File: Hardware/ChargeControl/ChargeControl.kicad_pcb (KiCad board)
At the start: 2 copper layers, 57 x 28 mm, 28 parts, among them J1 Conn_01x03, J2 Conn_01x04, J3 Conn_01x04, J4 Conn_01x08, Q1 Q-FET-N-SSM3K36MFV, U1 74LVC1G14, U2 MCP602

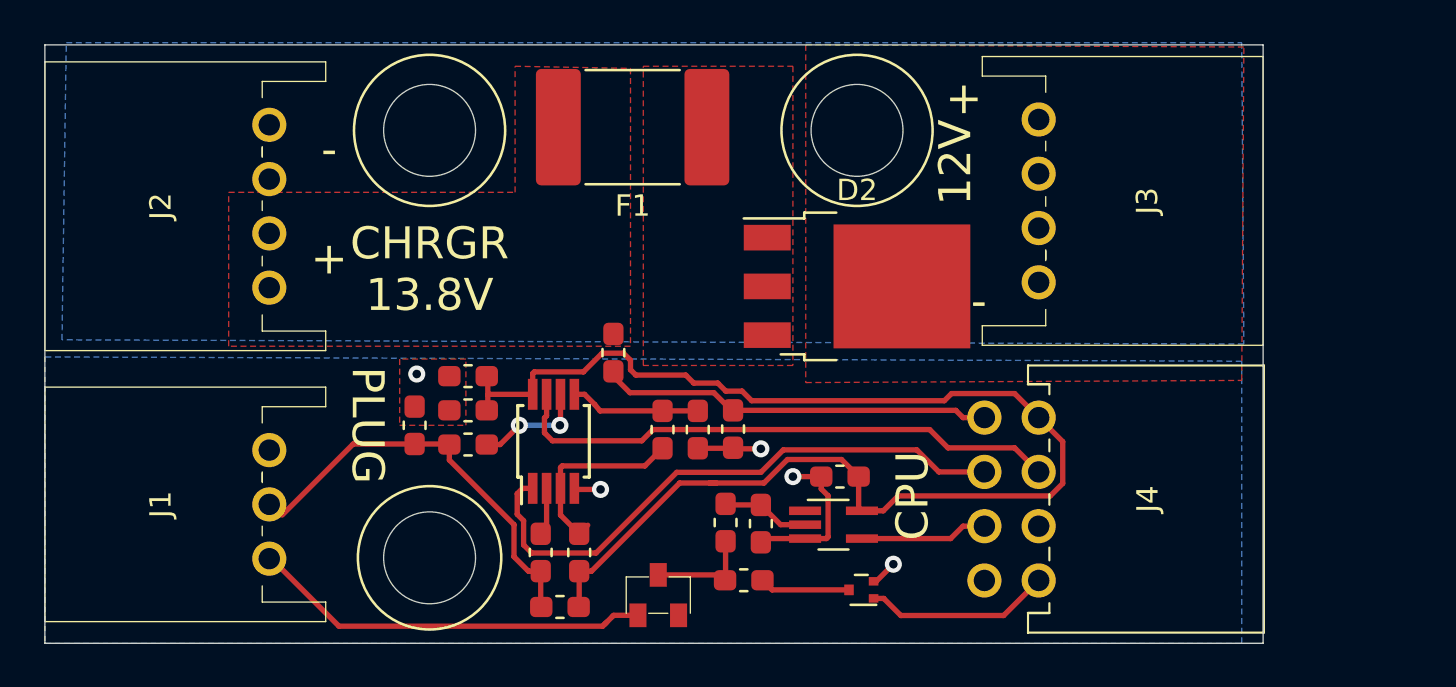
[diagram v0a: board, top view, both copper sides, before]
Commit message: Older PCB updates
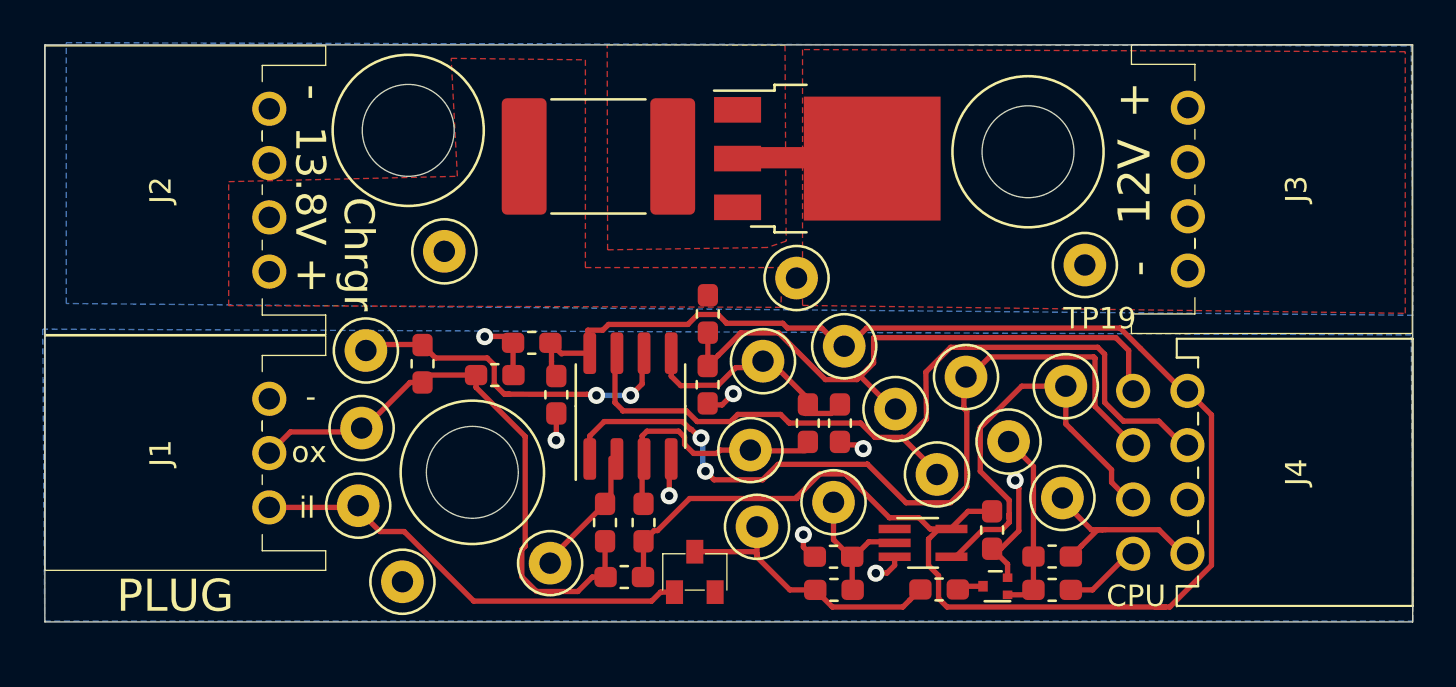
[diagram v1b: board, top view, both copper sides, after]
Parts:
- added R13: 3.3k, Resistor_SMD:R_0603_1608Metric_Pad1.05x0.95mm_HandSolder, F.Cu at (149.1, 84.9)
- added R14: 100k, Resistor_SMD:R_0603_1608Metric_Pad1.05x0.95mm_HandSolder, F.Cu at (149.1, 86.5)
- added TP1: TestPoint, TestPoint:TestPoint_Loop_D2.50mm_Drill1.0mm_LowProfile, F.Cu at (116.7, 82.6)
- added TP10: TestPoint, TestPoint:TestPoint_Loop_D2.50mm_Drill1.0mm_LowProfile, F.Cu at (125.6, 85.2)
- added TP11: TestPoint, TestPoint:TestPoint_Loop_D2.50mm_Drill1.0mm_LowProfile, F.Cu at (117.0, 75.3)
- added TP12: TestPoint, TestPoint:TestPoint_Loop_D2.50mm_Drill1.0mm_LowProfile, F.Cu at (145.1, 76.5)
- added TP13: TestPoint, TestPoint:TestPoint_Loop_D2.50mm_Drill1.0mm_LowProfile, F.Cu at (143.7, 81.1)
- added TP14: TestPoint, TestPoint:TestPoint_Loop_D2.50mm_Drill1.0mm_LowProfile, F.Cu at (139.4, 75.1)
- added TP15: TestPoint, TestPoint:TestPoint_Loop_D2.50mm_Drill1.0mm_LowProfile, F.Cu at (118.7, 86.1)
- added TP16: TestPoint, TestPoint:TestPoint_Loop_D2.50mm_Drill1.0mm_LowProfile, F.Cu at (135.0, 80.0)
- added TP17: TestPoint, TestPoint:TestPoint_Loop_D2.50mm_Drill1.0mm_LowProfile, F.Cu at (135.6, 75.8)
- added TP18: TestPoint, TestPoint:TestPoint_Loop_D2.50mm_Drill1.0mm_LowProfile, F.Cu at (137.2, 71.9)
- added TP19: TestPoint, TestPoint:TestPoint_Loop_D2.50mm_Drill1.0mm_LowProfile, F.Cu at (150.7, 71.3)
- added TP2: TestPoint, TestPoint:TestPoint_Loop_D2.50mm_Drill1.0mm_LowProfile, F.Cu at (149.6, 82.2)
- added TP3: TestPoint, TestPoint:TestPoint_Loop_D2.50mm_Drill1.0mm_LowProfile, F.Cu at (147.1, 79.6)
- added TP4: TestPoint, TestPoint:TestPoint_Loop_D2.50mm_Drill1.0mm_LowProfile, F.Cu at (135.3, 83.5)
- added TP5: TestPoint, TestPoint:TestPoint_Loop_D2.50mm_Drill1.0mm_LowProfile, F.Cu at (116.8, 78.9)
- added TP6: TestPoint, TestPoint:TestPoint_Loop_D2.50mm_Drill1.0mm_LowProfile, F.Cu at (138.9, 82.4)
- added TP7: TestPoint, TestPoint:TestPoint_Loop_D2.50mm_Drill1.0mm_LowProfile, F.Cu at (120.7, 70.7)
- added TP8: TestPoint, TestPoint:TestPoint_Loop_D2.50mm_Drill1.0mm_LowProfile, F.Cu at (141.8, 78.0)
- added TP9: TestPoint, TestPoint:TestPoint_Loop_D2.50mm_Drill1.0mm_LowProfile, F.Cu at (149.8, 77.0)
- U2: footprint Package_SO:MSOP-8_3x3mm_P0.65mm -> Package_SO:SOIC-8_3.9x4.9mm_P1.27mm
- moved R1 9.15 mm to (143.8, 86.5)
- moved H2 8.06 mm to (148.0, 66.0)
- moved C1 7.55 mm to (146.3, 83.7), turned to 270 degrees
- moved J4 7.07 mm to (155.5, 81.0)
- moved J3 7.00 mm to (155.5, 67.8)
- moved R11 6.81 mm to (137.7, 78.7)
- moved R12 6.66 mm to (139.2, 78.7)
- moved Q1 6.27 mm to (146.5, 86.3)
- moved D2 6.14 mm to (138.6, 66.3)
- moved R2 5.97 mm to (138.9, 86.5), turned to 180 degrees
- moved R5 4.78 mm to (133.0, 73.6)
- moved H3 4.47 mm to (122.0, 81.0)
- moved R4 4.43 mm to (123.0, 76.5), turned to 180 degrees
- moved R9 4.34 mm to (119.7, 75.9), turned to 90 degrees
- moved U1 4.28 mm to (143.1, 84.3)
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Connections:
- Q1 pad 1: /PILOT_EV_CHARGE -> Net-(Q1-Pad1)
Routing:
- net +3V3: track 63.3 -> 83.0 mm
- net /PILOT_OUT: track 5.97 -> 19.9 mm
- net /PROXIMITY_0: track 26.2 -> 38.4 mm
- net Net-(R9-Pad2): track 5.22 -> 16.4 mm
- net /PROXIMITY_1: track 27.7 -> 38.8 mm, vias 0 -> 2
- net /CHARGER_POWER_SENSE: track 18.6 -> 28.7 mm
- net Net-(Q1-Pad1): track 0.00 -> 8.73 mm
- net Net-(D1-Pad3): track 5.06 -> 13.3 mm
- net /PLUG_PROXIMITY: track 19.5 -> 27.8 mm
- net GND: track 12.9 -> 20.5 mm, vias 5 -> 8
- net +12V: track 0.00 -> 6.30 mm
- net /1.4V: track 6.11 -> 10.9 mm
- net Net-(R8-Pad2): track 2.24 -> 5.69 mm
- net Net-(Q1-Pad3): track 4.51 -> 1.24 mm
- net /PLUG_PILOT: track 18.1 -> 21.0 mm
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- removed copper zone on F.Cu, net GND
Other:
- board size 57 x 28 mm -> 64 x 27 mm
- rule trace_min: 0.2 -> 0.1524
- board text added: "13.8V"
- board text added: "Charger 13.8V"
- board text added: "Chrgr"
- board text added: "Plug"
- board text added: "System 12V"
- board text added: "Type 2 EV Interface Version 2"
- board text added: "il"
- board text added: "ox"
- board text removed: "CHRGR 13.8V"
- board text removed: "Type 2 EV Interface Version 1"
